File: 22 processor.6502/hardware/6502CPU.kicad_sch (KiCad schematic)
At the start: 22 parts, among them J4 RES SEL, SW1 RESET, U1 74LS04, U13 CPU CLOCK, U15 DS1233, U23 W65C02SxPL, U4 74LS07, U5 27C010, U7 74LS14

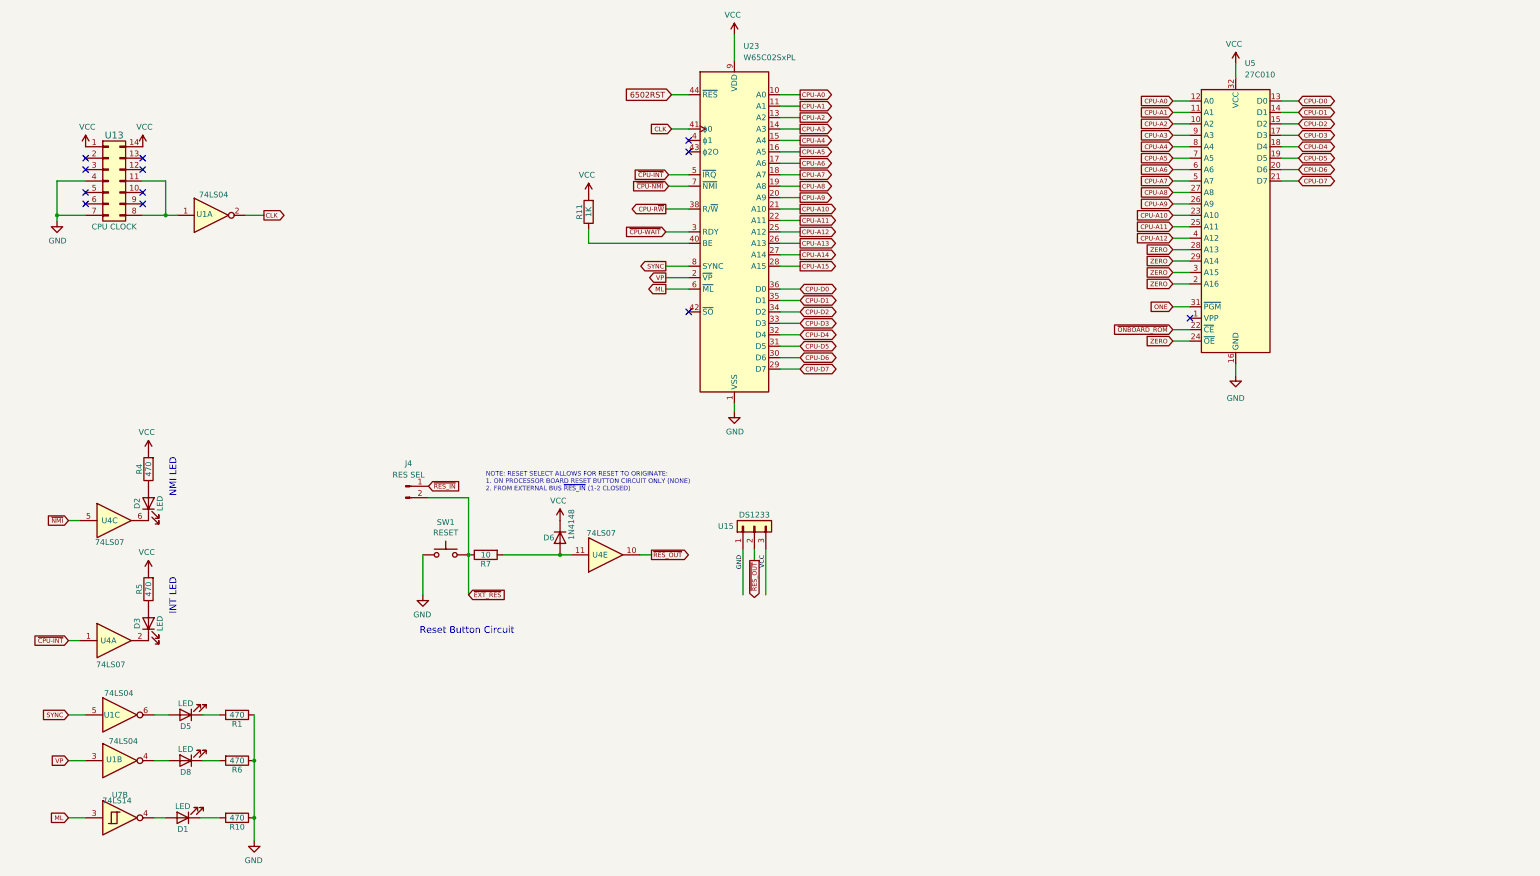
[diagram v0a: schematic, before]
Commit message: duodyne 6502 work
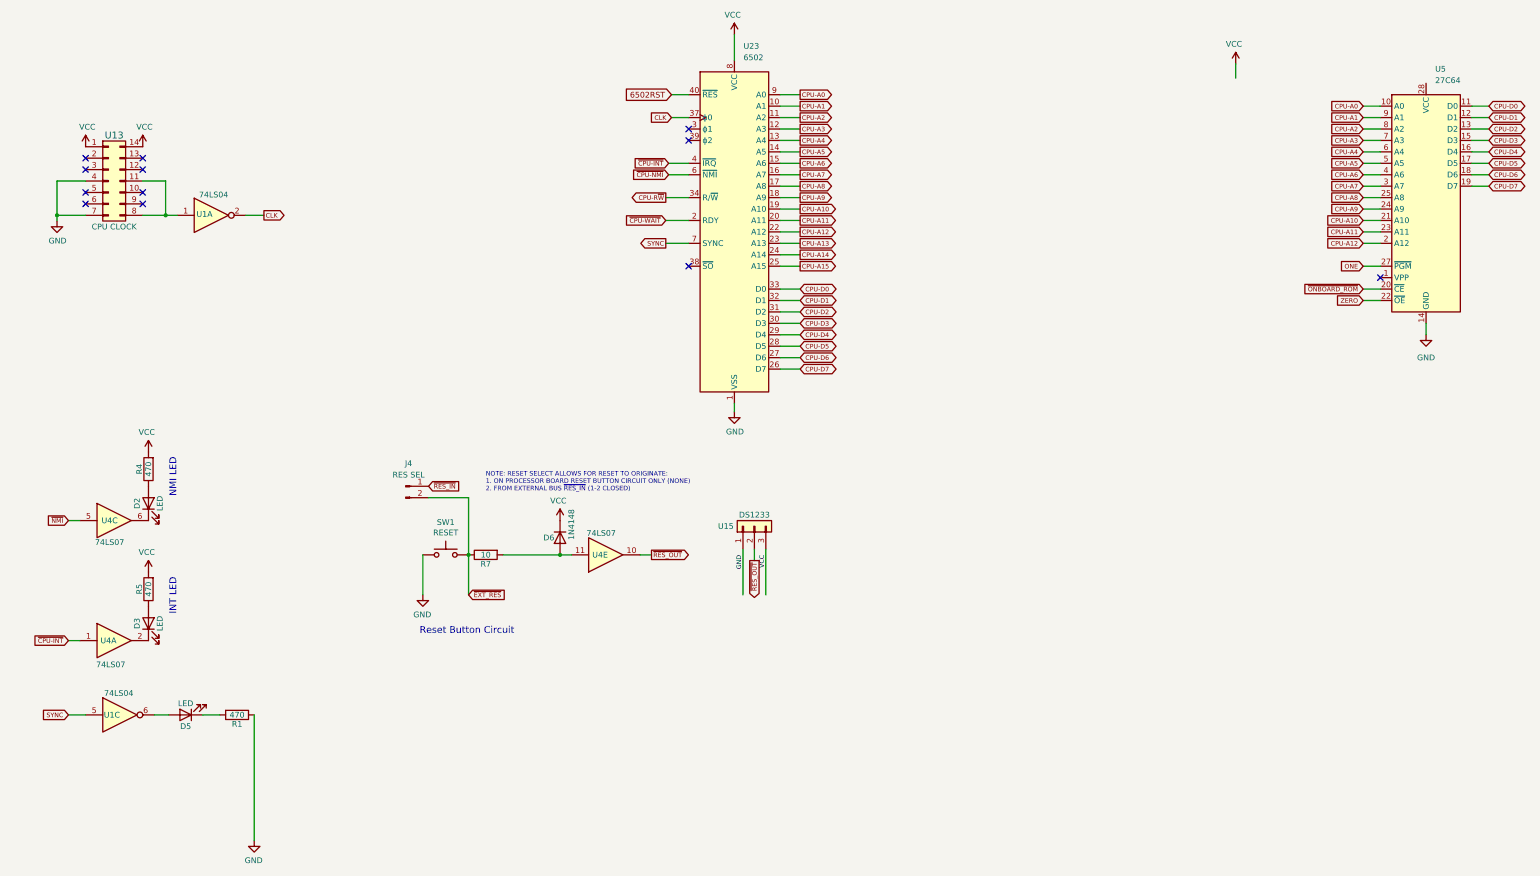
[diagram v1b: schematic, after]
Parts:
- removed D1, D8: LED, LED_THT:LED_D3.0mm_Horizontal_O3.81mm_Z2.0mm, symbol Device:LED
- removed R10, R6: 470, Resistor_THT:R_Axial_DIN0207_L6.3mm_D2.5mm_P7.62mm_Horizontal, symbol Device:R
- removed R11: 1K, Resistor_THT:R_Axial_DIN0207_L6.3mm_D2.5mm_P7.62mm_Horizontal, symbol Device:R
- removed unit 2 of U1
- removed U23: W65C02SxPL, Package_LCC:PLCC-44_THT-Socket, symbol 65xx-library:W65C02SxPL
- removed U5: 27C010, Package_DIP:DIP-32_W15.24mm_Socket_LongPads, symbol Memory_EPROM:27C010
- removed U7: 74LS14, Package_DIP:DIP-14_W7.62mm_Socket_LongPads, symbol 74xx:74LS14
- added U23: 6502, Package_DIP:DIP-40_W15.24mm_Socket_LongPads, symbol 65xxx-library:6502
- added U5: 27C64, Package_DIP:DIP-28_W15.24mm, symbol Memory_EPROM:27C64
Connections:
- net 6502RST: now also U23.40 (~{RES})
- net CLK: now also U23.37 (ϕ0)
- net CPU-A0: now also U23.9 (A0), U5.10 (A0)
- net CPU-A1: now also U23.10 (A1), U5.9 (A1)
- net CPU-A10: now also U23.19 (A10), U5.21 (A10)
- net CPU-A11: now also U23.20 (A11), U5.23 (A11)
- net CPU-A12: now also U23.22 (A12), U5.2 (A12)
- net CPU-A13: now also U23.23 (A13)
- net CPU-A14: now also U23.24 (A14)
- net CPU-A15: now also U23.25 (A15)
- net CPU-A2: now also U23.11 (A2), U5.8 (A2)
- net CPU-A3: now also U23.12 (A3), U5.7 (A3)
- net CPU-A4: now also U23.13 (A4), U5.6 (A4)
- net CPU-A5: now also U23.14 (A5), U5.5 (A5)
- net CPU-A6: now also U23.15 (A6), U5.4 (A6)
- net CPU-A7: now also U23.16 (A7), U5.3 (A7)
- net CPU-A8: now also U23.17 (A8), U5.25 (A8)
- net CPU-A9: now also U23.18 (A9), U5.24 (A9)
- net CPU-D0: now also U23.33 (D0), U5.11 (D0)
- net CPU-D1: now also U23.32 (D1), U5.12 (D1)
- net CPU-D2: now also U23.31 (D2), U5.13 (D2)
- net CPU-D3: now also U23.30 (D3), U5.15 (D3)
- net CPU-D4: now also U23.29 (D4), U5.16 (D4)
- net CPU-D5: now also U23.28 (D5), U5.17 (D5)
- net CPU-D6: now also U23.27 (D6), U5.18 (D6)
- net CPU-D7: now also U23.26 (D7), U5.19 (D7)
- net CPU-R~{W}: now also U23.34 (R/~{W})
- net GND: now also U23.1 (VSS), U23.21 (VSS), U5.14 (GND)
- net ONE: now also U5.27 (~{PGM})
- net SYNC: now also U23.7 (SYNC)
- net VCC: now also U23.8 (VCC)
- net ZERO: now also U5.22 (~{OE})
- net ~{CPU-INT}: now also U23.4 (~{IRQ})
- net ~{CPU-NMI}: now also U23.6 (~{NMI})
- net ~{CPU-WAIT}: now also U23.2 (RDY)
- net ~{ONBOARD_ROM}: now also U5.20 (~{CE})
